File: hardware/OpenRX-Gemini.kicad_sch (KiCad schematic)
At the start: 0 parts

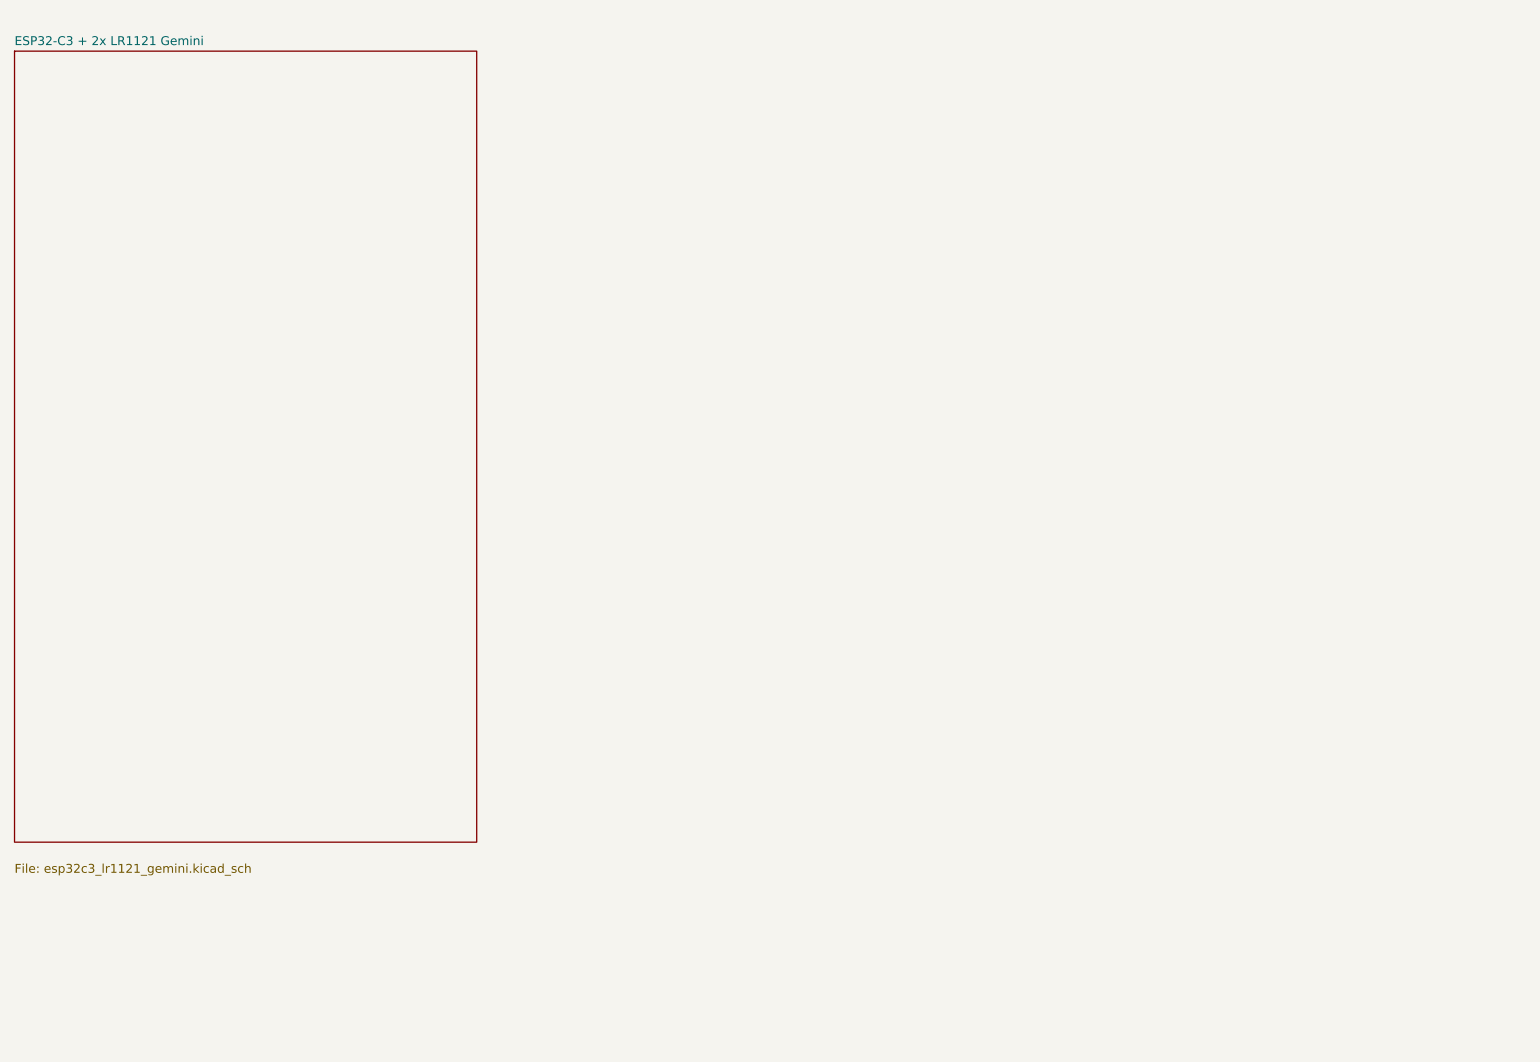
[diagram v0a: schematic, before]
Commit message: gemini initial
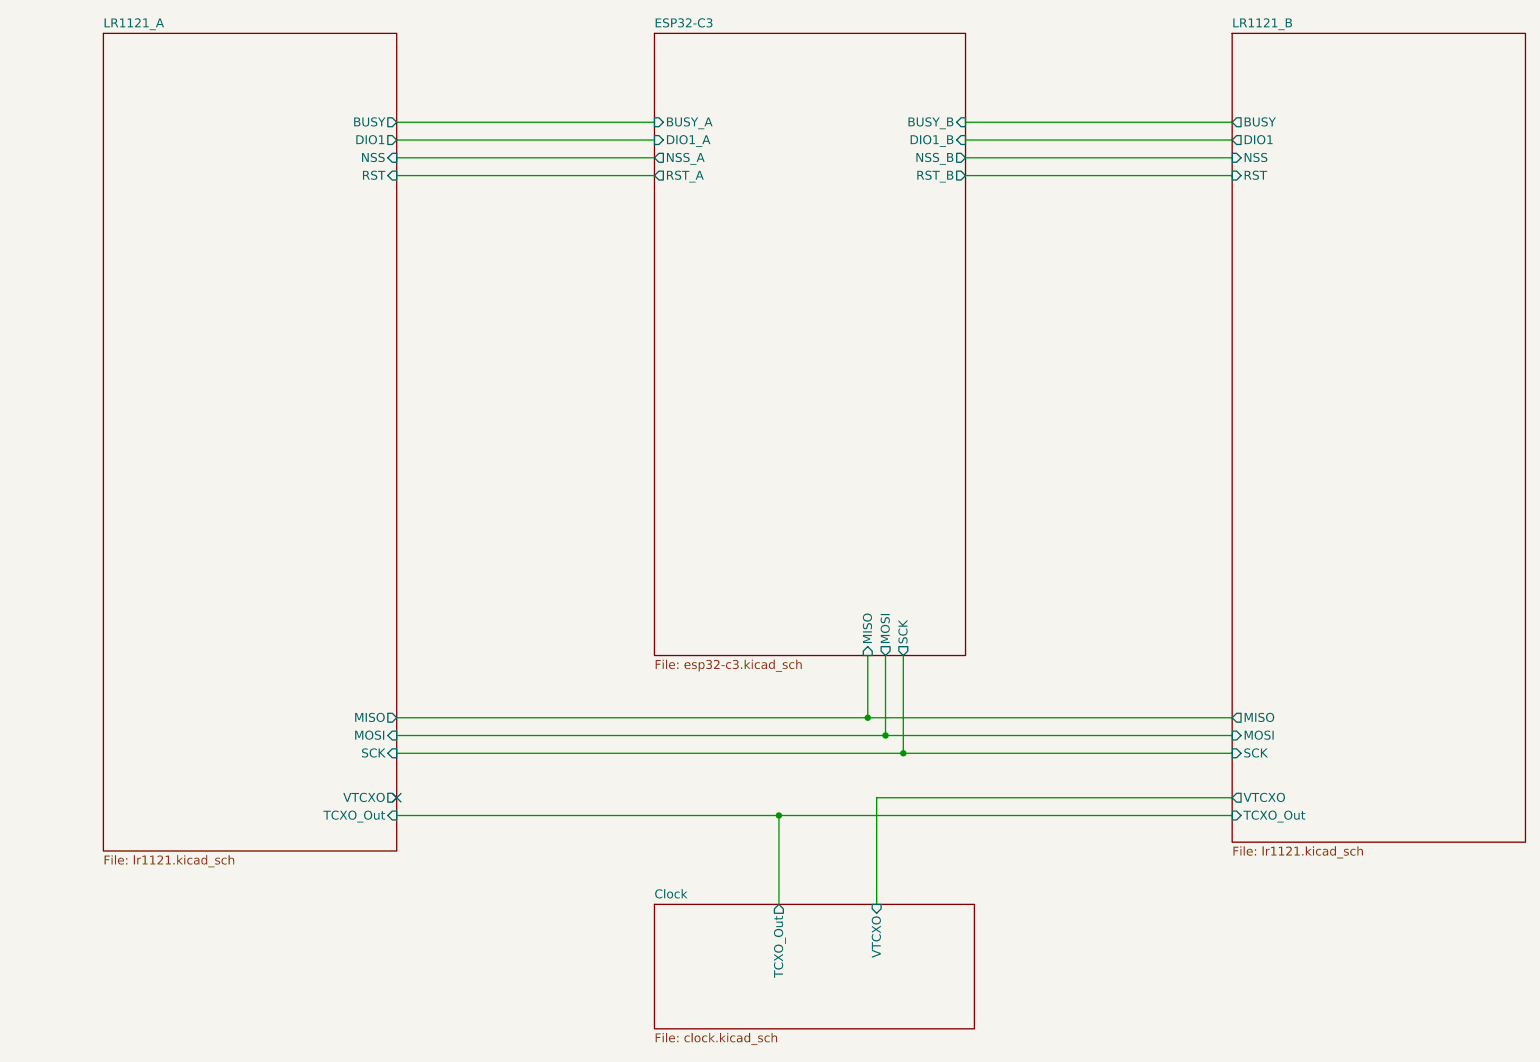
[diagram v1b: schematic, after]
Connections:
- no-connect marks 0 -> 1
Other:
- removed sheet ESP32-C3 + 2x LR1121 Gemini
- added sheet Clock (clock.kicad_sch)
- added sheet ESP32-C3 (esp32-c3.kicad_sch)
- added sheet LR1121_A (lr1121.kicad_sch)
- added sheet LR1121_B (lr1121.kicad_sch)
